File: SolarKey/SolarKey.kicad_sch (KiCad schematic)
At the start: 95 parts, among them U1 ESP32-WROOM-32

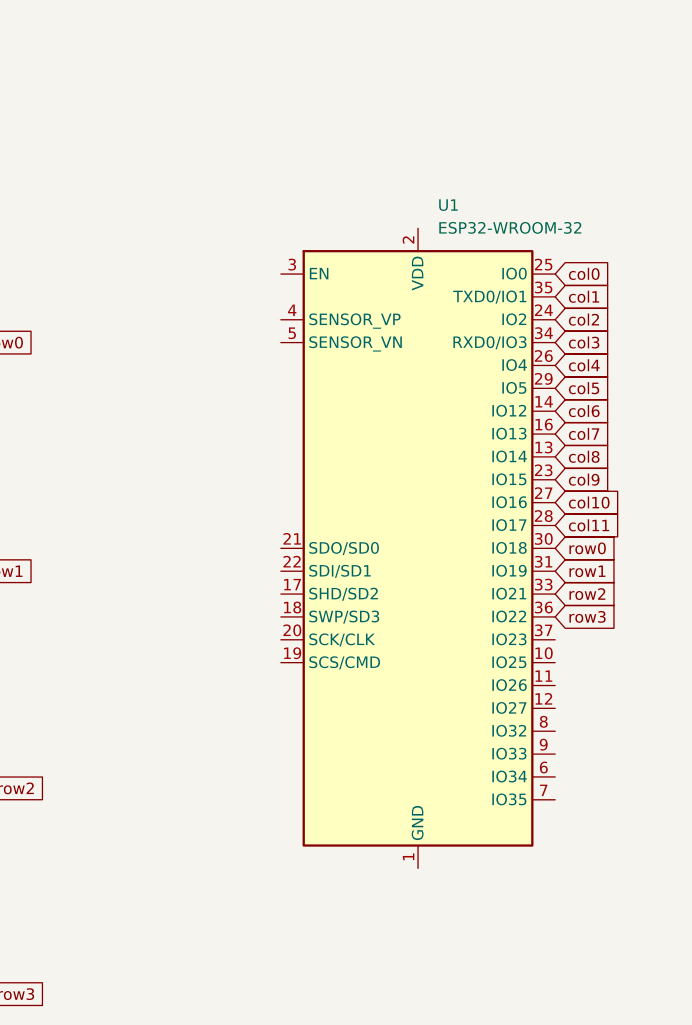
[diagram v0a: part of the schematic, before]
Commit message: Initial commit
Add initial project files and setup.
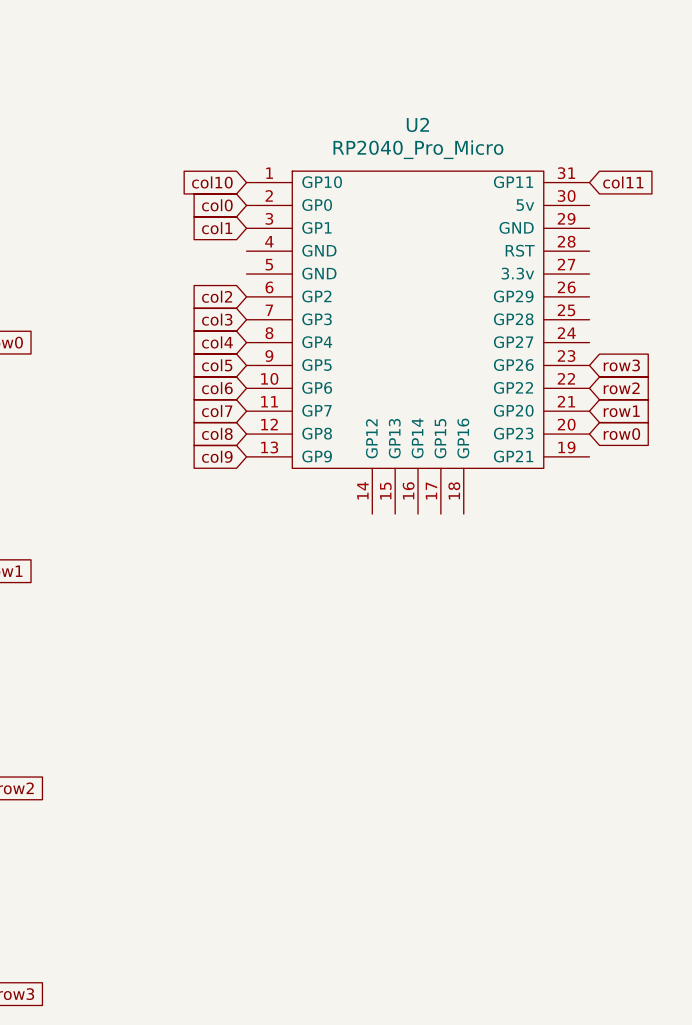
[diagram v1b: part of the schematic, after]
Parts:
- removed U1: ESP32-WROOM-32, RF_Module:ESP32-WROOM-32, symbol RF_Module:ESP32-WROOM-32
- added U2: RP2040_Pro_Micro, ScottoKeebs_MCU:RP2040_Pro_Micro, symbol ScottoKeebs:MCU_RP2040_Pro_Micro
- D1, D10, D11, D12, D13, D14, D15, D16, D17, D18, D19, D2, D20, D21, D22, D23, D24, D25, D26, D27, D28, D29, D3, D30, D31, D32, D33, D34, D35, D36, D37, D38, D39, D4, D40, D41, D42, D43, D44, D45, D46, D47, D5, D6, D7, D8, D9: footprint (none) -> Diode_SMD:D_SOD-123
- S1, S10, S11, S12, S13, S14, S15, S16, S17, S18, S19, S2, S20, S21, S22, S23, S24, S25, S26, S27, S28, S29, S3, S30, S31, S32, S33, S34, S35, S36, S37, S38, S39, S4, S40, S41, S42, S43, S44, S45, S46, S47, S5, S6, S7, S8, S9: footprint (none) -> KS33:SW_Gateron_LowProfile_HotSwap_PTH
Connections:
- net col0: now also U2.2 (GP0)
- net col1: now also U2.3 (GP1)
- net col10: now also U2.1 (GP10)
- net col11: now also U2.31 (GP11)
- net col2: now also U2.6 (GP2)
- net col3: now also U2.7 (GP3)
- net col4: now also U2.8 (GP4)
- net col5: now also U2.9 (GP5)
- net col6: now also U2.10 (GP6)
- net col7: now also U2.11 (GP7)
- net col8: now also U2.12 (GP8)
- net col9: now also U2.13 (GP9)
- net row0: now also U2.20 (GP23)
- net row1: now also U2.21 (GP20)
- net row2: now also U2.22 (GP22)
- net row3: now also U2.23 (GP26)
